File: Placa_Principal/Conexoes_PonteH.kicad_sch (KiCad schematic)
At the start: 6 parts, among them J2 Conn_01x02, J3 Conn_01x02, J4 Conn_01x02, J5 Conn_01x02, U4 L298N MODULE, U5 L298N MODULE

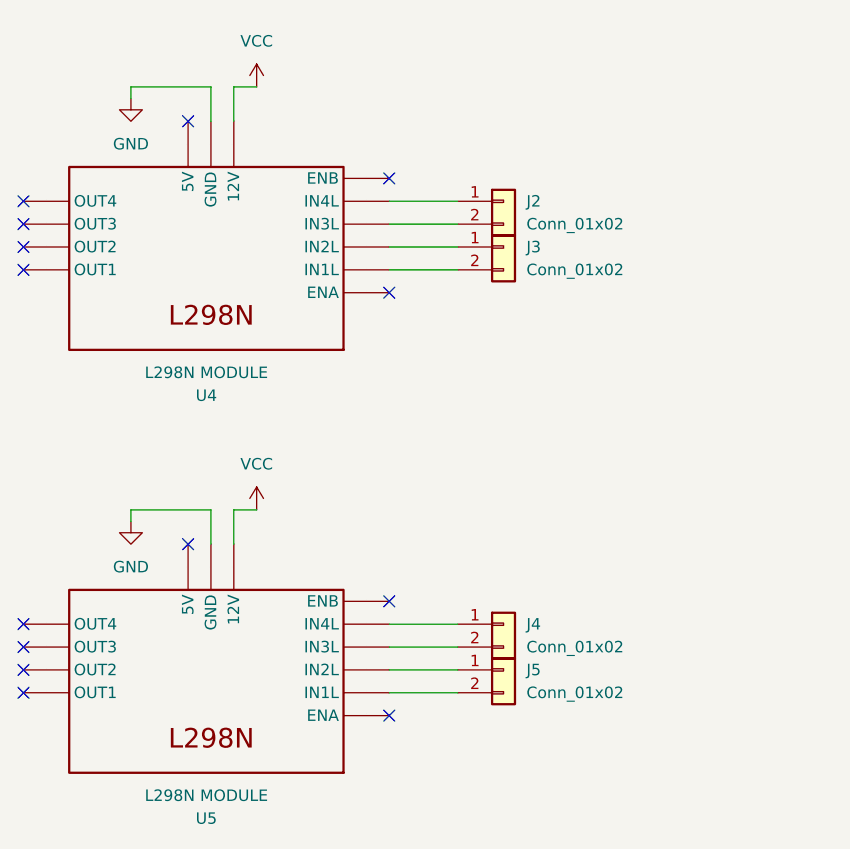
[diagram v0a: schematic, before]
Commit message: Segundo commit
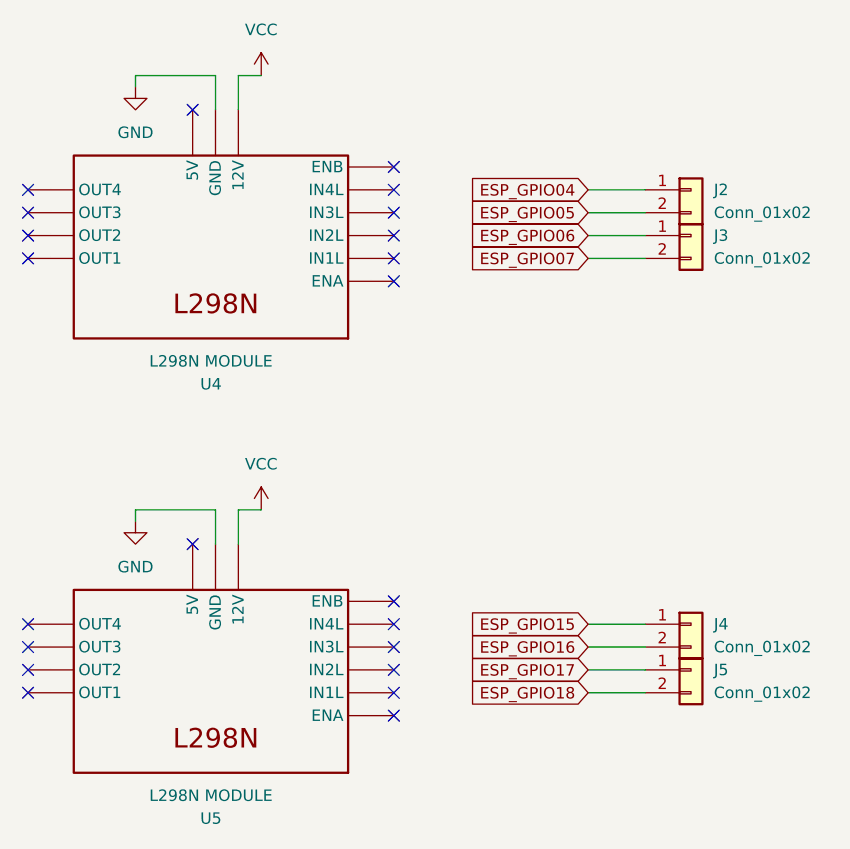
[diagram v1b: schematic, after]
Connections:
- net at U4.2 (IN2L): no longer J3.1 (Pin_1)
- net at U4.1 (IN1L): no longer J3.2 (Pin_2)
- net at U5.1 (IN1L): no longer J5.2 (Pin_2)
- net at U5.2 (IN2L): no longer J5.1 (Pin_1)
- net at U5.3 (IN3L): no longer J4.2 (Pin_2)
- net at U5.4 (IN4L): no longer J4.1 (Pin_1)
- net at U4.3 (IN3L): no longer J2.2 (Pin_2)
- net at U4.4 (IN4L): no longer J2.1 (Pin_1)
- new net ESP_GPIO04: J2.1 (Pin_1)
- new net ESP_GPIO05: J2.2 (Pin_2)
- new net ESP_GPIO06: J3.1 (Pin_1)
- new net ESP_GPIO07: J3.2 (Pin_2)
- new net ESP_GPIO15: J4.1 (Pin_1)
- new net ESP_GPIO16: J4.2 (Pin_2)
- new net ESP_GPIO17: J5.1 (Pin_1)
- new net ESP_GPIO18: J5.2 (Pin_2)
- no-connect marks 14 -> 22
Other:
- moved on the sheet: J2, J3, J4, J5, U4, U5
